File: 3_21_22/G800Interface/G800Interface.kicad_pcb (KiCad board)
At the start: 2 copper layers, 35 parts, among them J1 11pin G800 Conn., J2 USB_C_Receptacle_USB2.0, U1 FT232RL

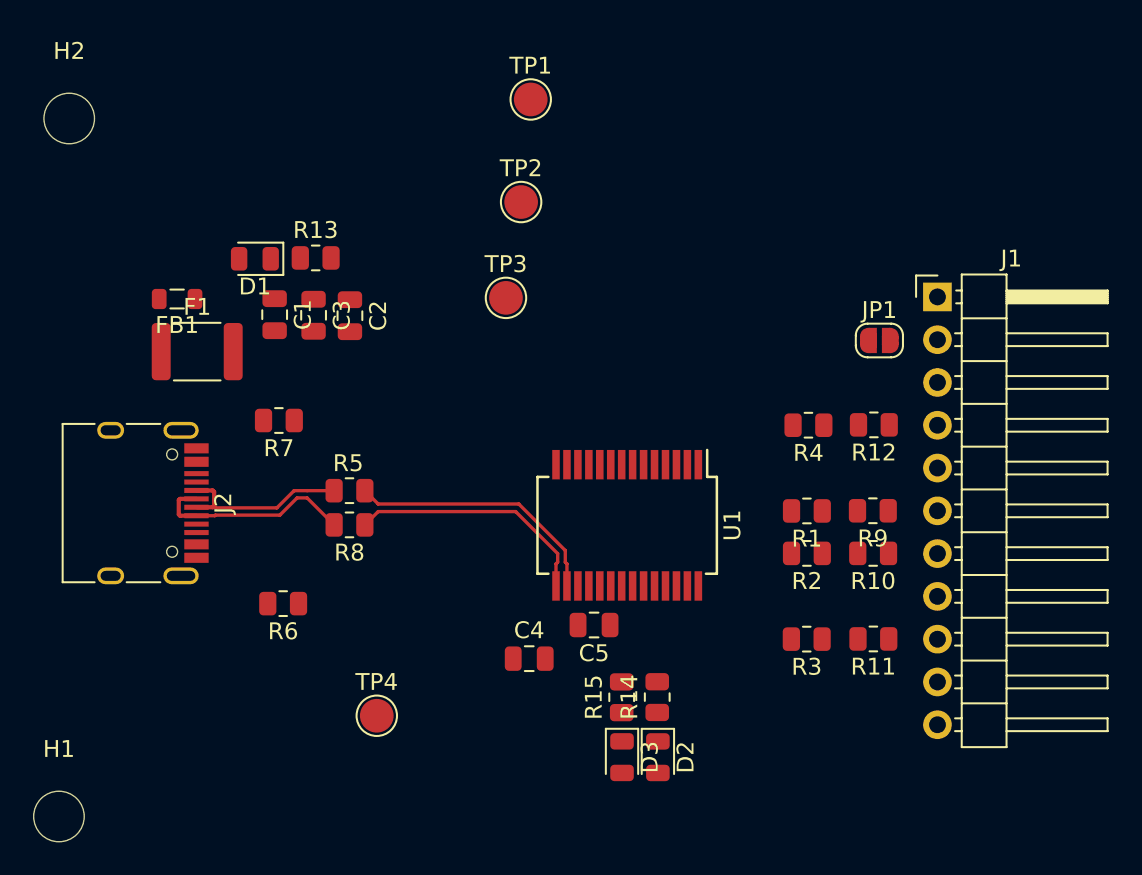
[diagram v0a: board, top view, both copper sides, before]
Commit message: finished G800
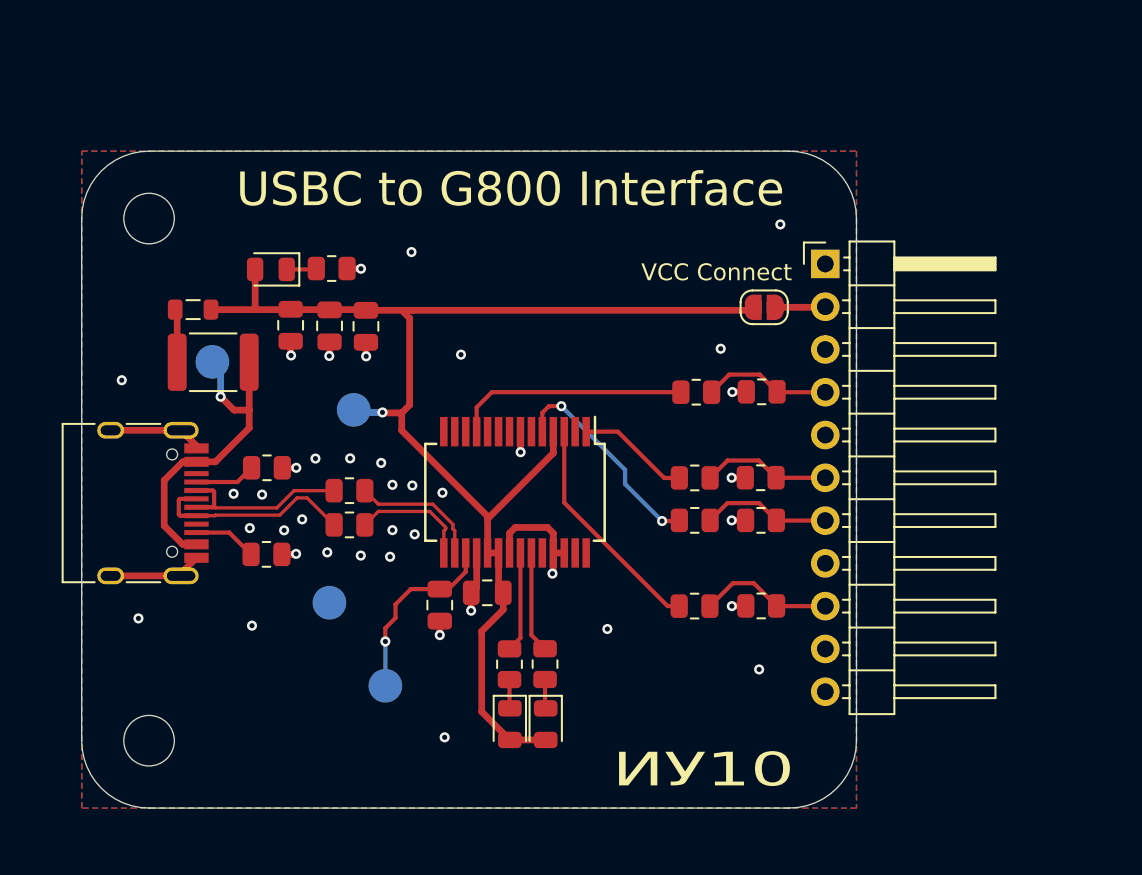
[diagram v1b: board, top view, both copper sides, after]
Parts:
- TP1, TP2, TP3, TP4: moved to B.Cu
- moved TP3 24.1 mm to (99.0, 97.7)
- moved TP1 21.2 mm to (97.2, 81.4)
- moved TP2 20.6 mm to (88.8, 78.5)
- moved H2 7.60 mm to (85.0, 70.0)
- moved TP4 7.27 mm to (95.7, 92.8)
- moved JP1 7.12 mm to (121.5, 75.3)
- moved H1 6.99 mm to (85.0, 101.0)
- moved R1 6.94 mm to (117.4, 85.4)
- moved R2 6.94 mm to (117.4, 87.9)
- moved D2 6.94 mm to (108.5, 100.0)
- moved D3 6.94 mm to (106.4, 100.0)
- moved J1 6.94 mm to (125.1, 72.7)
- moved U1 6.94 mm to (106.7, 86.3)
- moved R10 6.94 mm to (121.3, 87.9)
- moved R11 6.94 mm to (121.3, 93.0)
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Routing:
- net VCCIO: track 0.00 -> 76.8 mm, vias 0 -> 1
- net GND: track 0.00 -> 32.3 mm, vias 0 -> 40
- net VBUS: track 0.00 -> 19.6 mm, vias 0 -> 1
- net Net-(R4-Pad2): track 0.00 -> 13.9 mm
- net Net-(R3-Pad2): track 0.00 -> 13.6 mm
- net Net-(R2-Pad2): track 0.00 -> 12.8 mm, vias 0 -> 2
- net +3V3: track 0.00 -> 11.2 mm, vias 0 -> 1
- net CTSCalc: track 0.00 -> 7.98 mm
- net USBD-: track 15.5 -> 7.80 mm
- net TXDCalc: track 0.00 -> 7.69 mm
- net RXDCalc: track 0.00 -> 7.69 mm
- net USBD+: track 14.8 -> 7.09 mm
- net RTSCalc: track 0.00 -> 7.62 mm
- net Net-(R1-Pad2): track 0.00 -> 6.67 mm
- net TXLED: track 0.00 -> 6.02 mm
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- added copper zone on B.Cu, net GND
- added copper zone on F.Cu, net GND
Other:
- board outline added: 46 x 39 mm
- net class Default: via_dia 0.8 -> 0.6; via_drill 0.4 -> 0.3
- net class PWR added: clearance 0.2, trace_width 0.4, via_dia 0.6, via_drill 0.3
- board text added: "+3.3V"
- board text added: "+5V"
- board text added: "GND"
- board text added: "USBC to G800 Interface"
- board text added: "VBUS"
- board text added: "VCC Connect"
- board text added: "ИУ10"
